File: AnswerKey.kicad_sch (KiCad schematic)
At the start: 37 parts

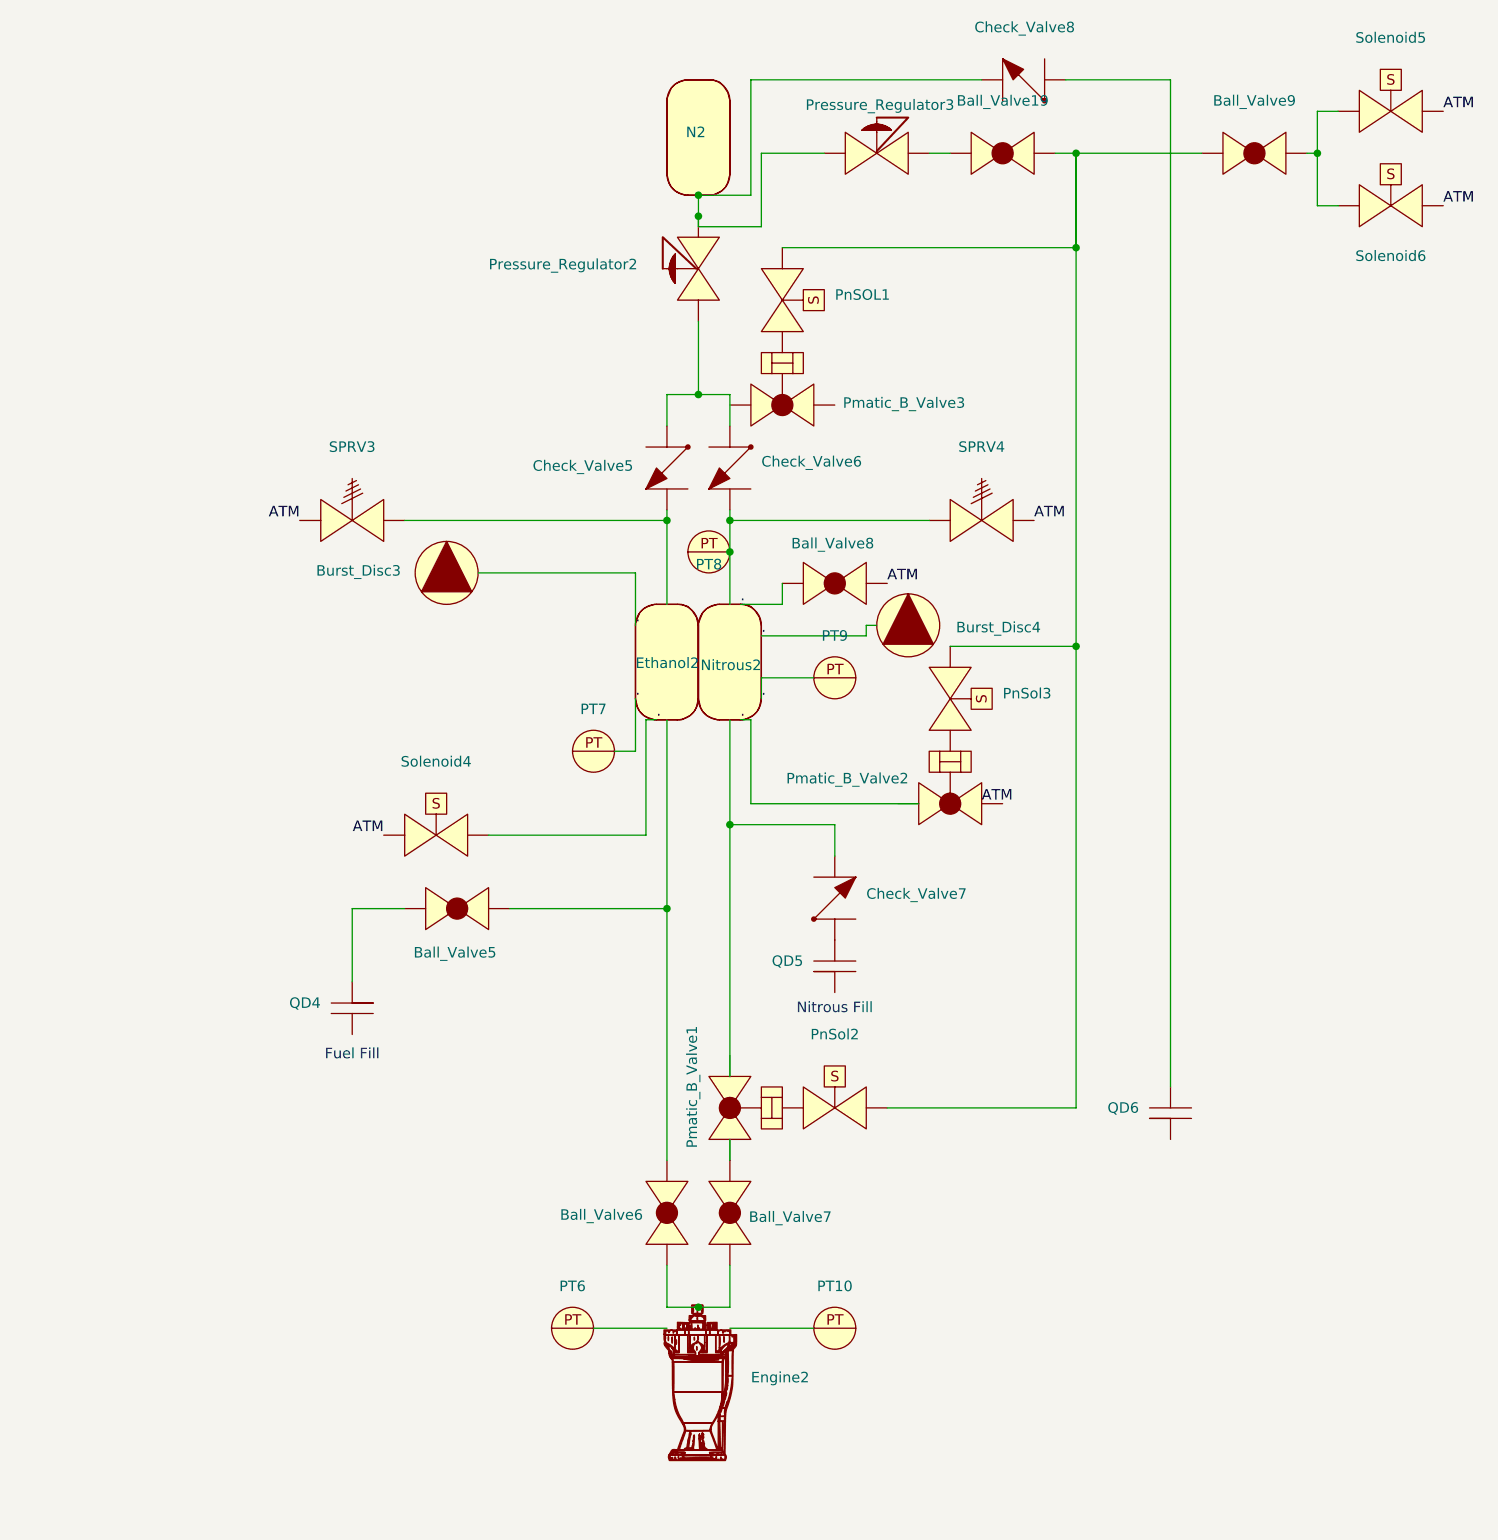
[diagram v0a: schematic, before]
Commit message: update, someone needs to finish adding torch igniter to answerkey, allow it im on holi
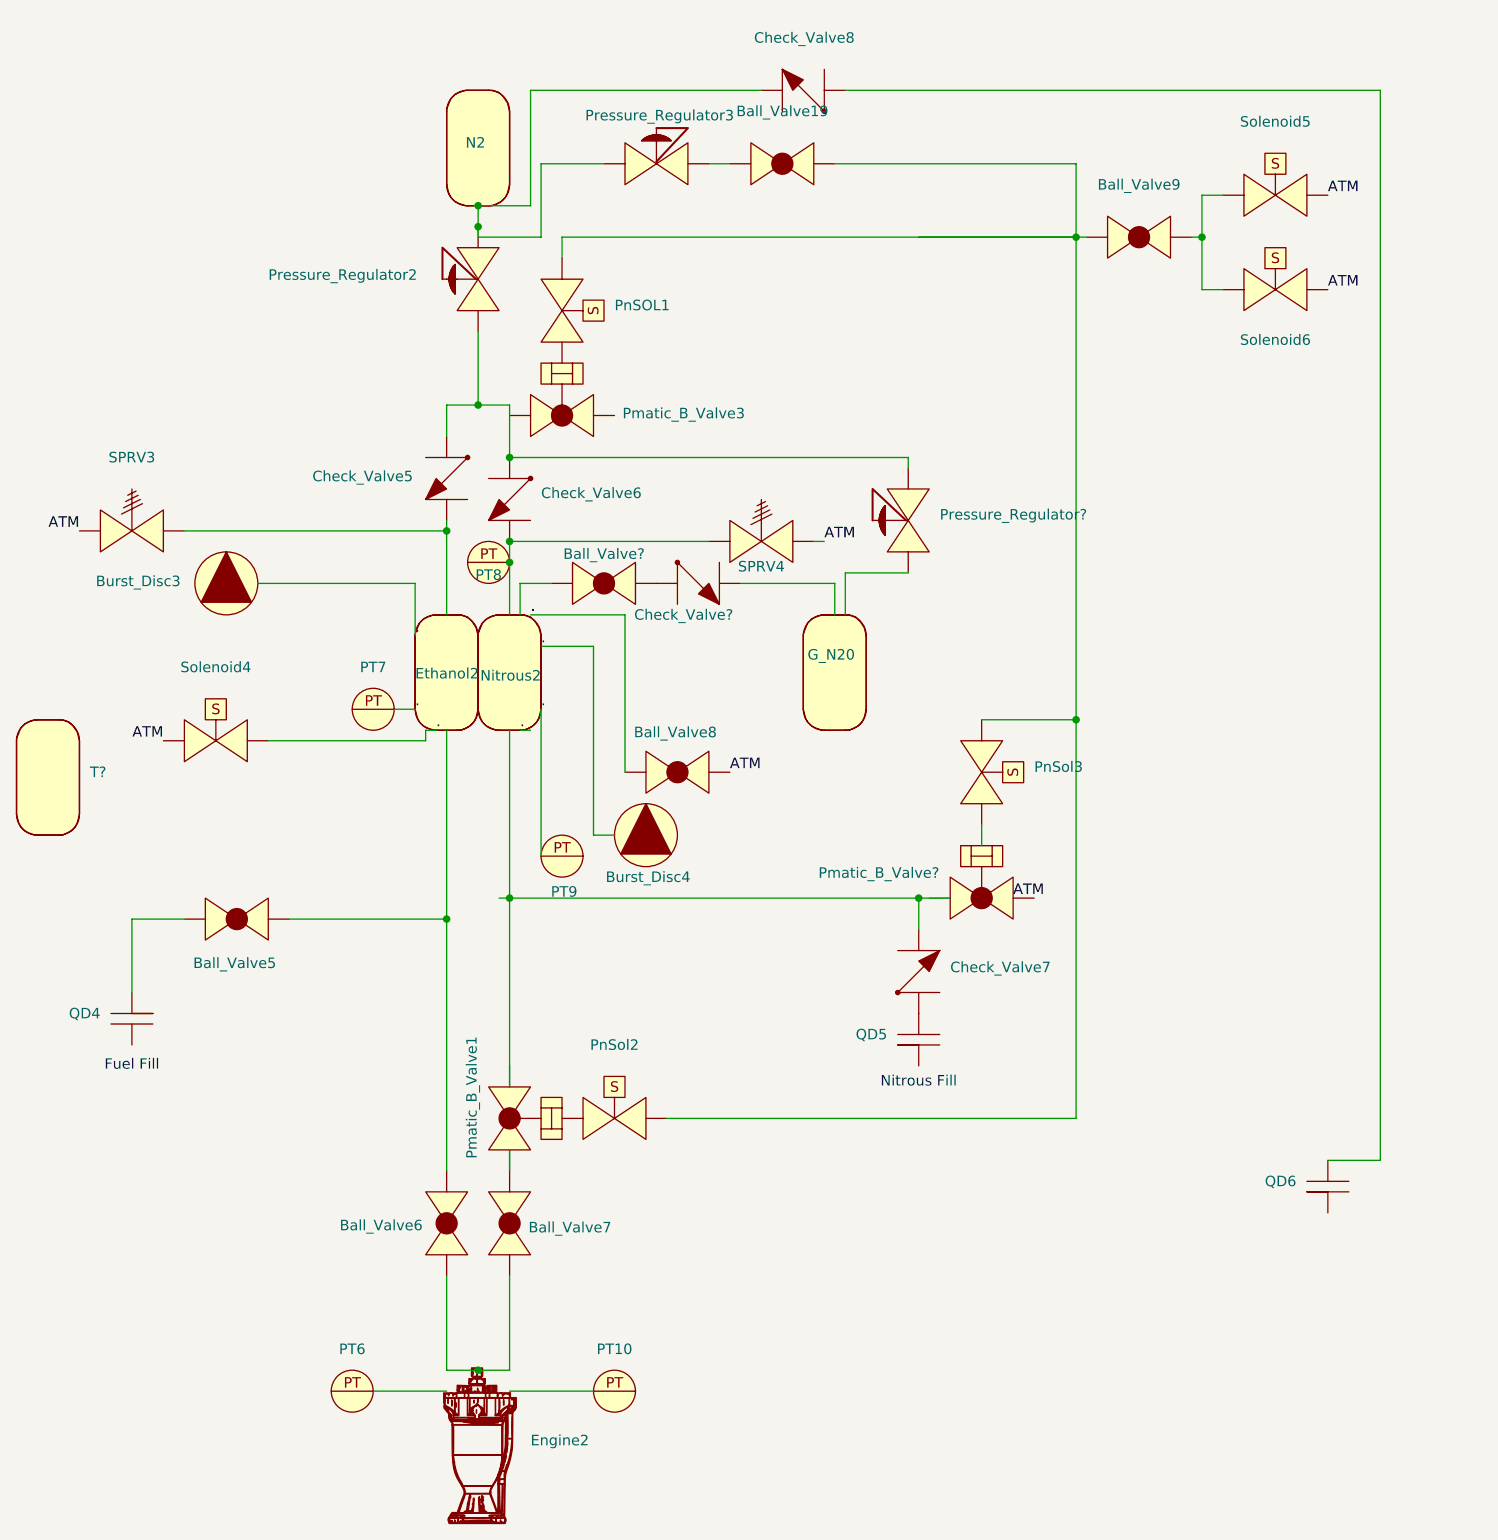
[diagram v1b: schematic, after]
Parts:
- removed Pmatic_B_Valve2: ~, symbol PID_symbols:Pneumatic_Rotary_Ball_Valve
- added Ball_Valve?: ~, symbol PID_symbols:Ball_Valve
- added Check_Valve?: ~, symbol PID_symbols:Check_Valve
- added G_N20, T?: ~, symbol PID_symbols:Tank
- added Pmatic_B_Valve?: ~, symbol PID_symbols:Pneumatic_Rotary_Ball_Valve
- added Pressure_Regulator?: ~, symbol PID_symbols:Pressure_Regulator
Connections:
- net ATM: now also Pmatic_B_Valve?.
- net at N2.: now also Check_Valve8., Pressure_Regulator2., Pressure_Regulator3.
- net at Engine2.: now also PT6.; no longer PT10.
- net at PT6.: no longer Engine2.
- net at Pmatic_B_Valve3.: now also PnSOL1.
- net at PnSOL1.: now also Ball_Valve19., Ball_Valve9., PnSol2., PnSol3.; no longer Pmatic_B_Valve3.
- net at QD5.: now also Check_Valve7.
- net at PT8.: now also Check_Valve6., Nitrous2., SPRV4.
- new net: Engine2., PT10.
- new net: Ball_Valve6., Ball_Valve7., Engine2.
- new net: Check_Valve5., Check_Valve6., Pressure_Regulator2., Pressure_Regulator?.
- new net: Check_Valve5., Ethanol2., SPRV3.
- new net: Check_Valve?., G_N20.
- new net: Ball_Valve?., Check_Valve?.
- new net: Pmatic_B_Valve?., PnSol3.
- new net: Check_Valve7., Nitrous2., Pmatic_B_Valve1., Pmatic_B_Valve?.
- new net: Ball_Valve9., Solenoid5., Solenoid6.
- now unconnected: Pmatic_B_Valve1.
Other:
- moved on the sheet: Ball_Valve19, Ball_Valve5, Ball_Valve6, Ball_Valve7, Ball_Valve8, Ball_Valve9, Burst_Disc3, Burst_Disc4, Check_Valve5, Check_Valve6, Check_Valve7, Check_Valve8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
